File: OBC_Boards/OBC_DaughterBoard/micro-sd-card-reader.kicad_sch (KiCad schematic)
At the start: 7 parts, among them J2 ST11S008V4HR2000

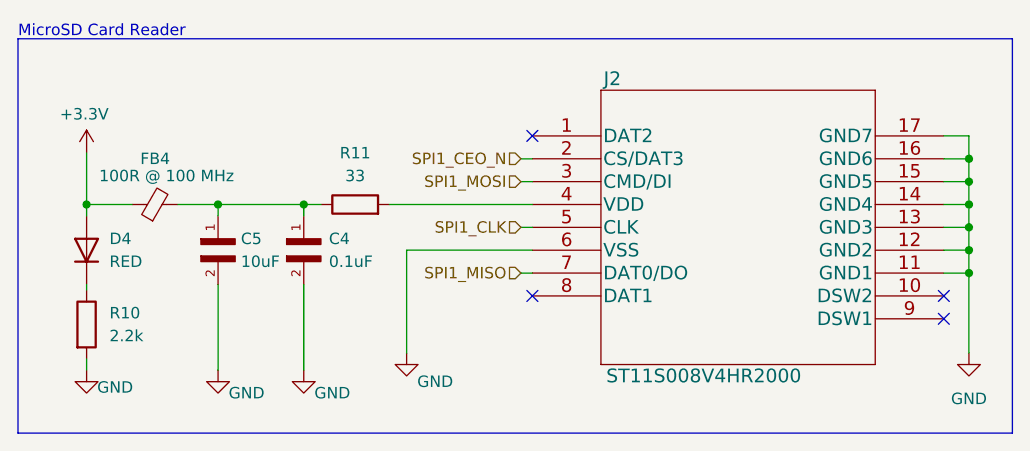
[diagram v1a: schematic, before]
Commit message: Layout completed
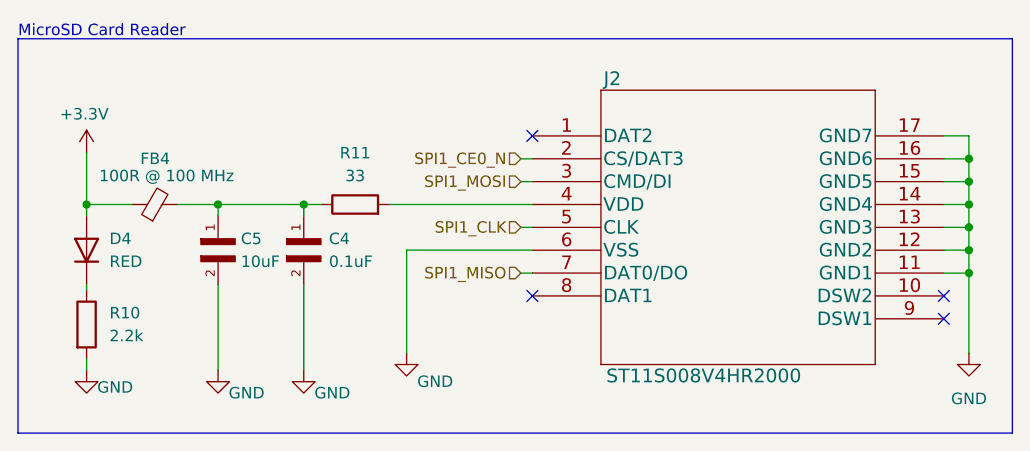
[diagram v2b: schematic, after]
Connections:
- net SPI1_CEO_N renamed SPI1_CE0_N
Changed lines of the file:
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@@
     (effects (font (size 1.27 1.27)) (justify right))
   )
-  (hierarchical_label "SPI1_CEO_N" (shape input) (at 137.16 88.265 180)
+  (hierarchical_label "SPI1_CE0_N" (shape input) (at 137.16 88.265 180)
     (effects (font (size 1.27 1.27)) (justify right))
   )
